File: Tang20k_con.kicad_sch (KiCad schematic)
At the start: 1 part

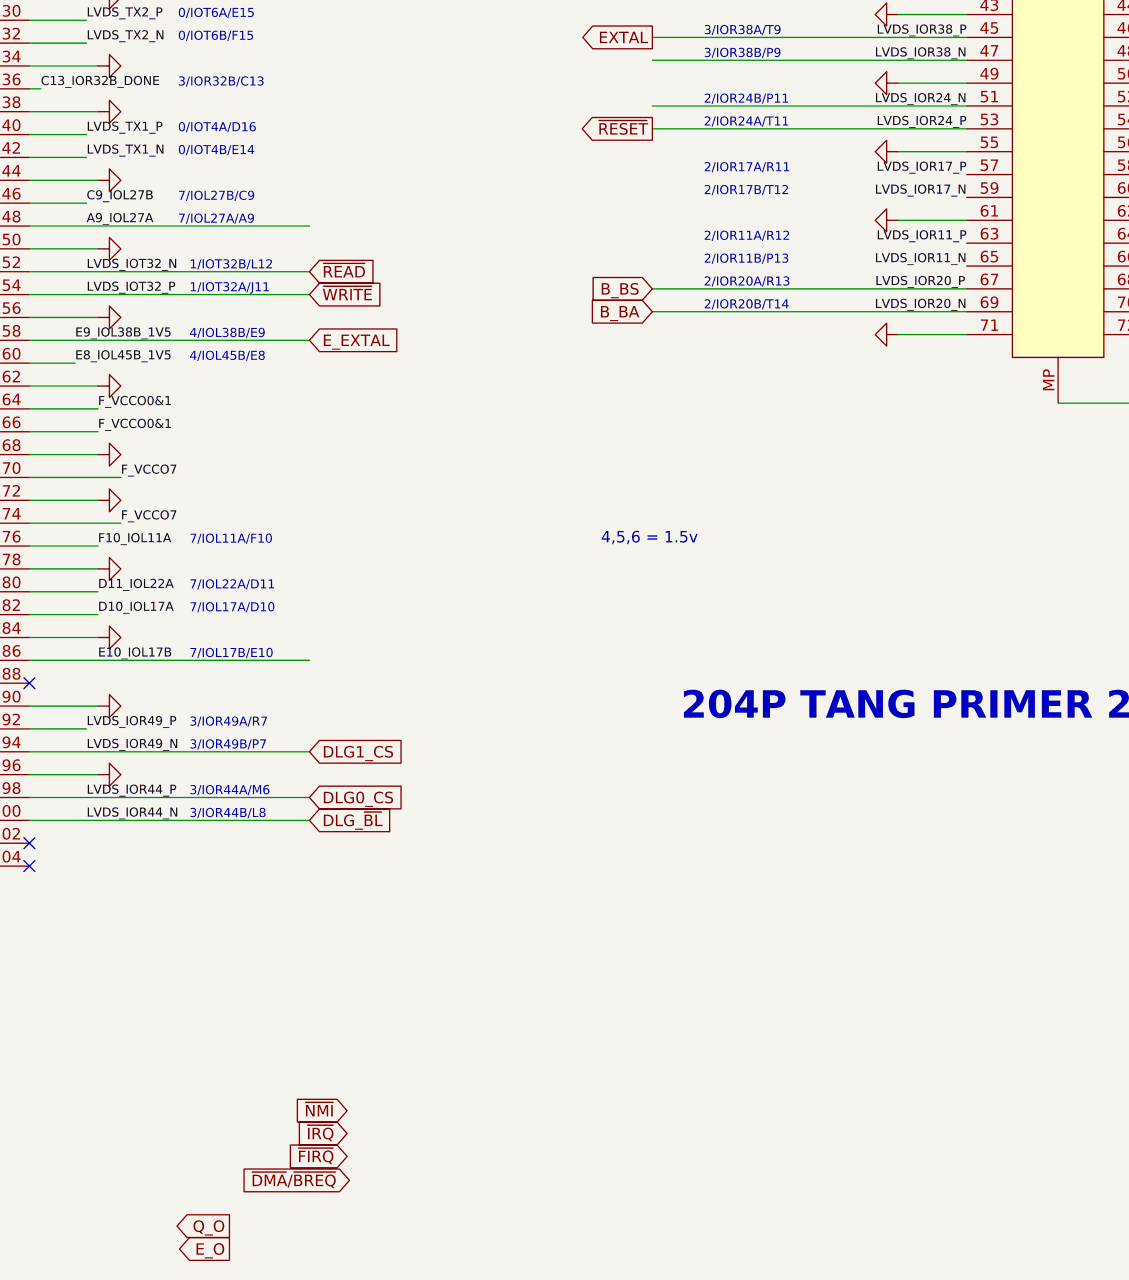
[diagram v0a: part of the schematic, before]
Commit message: WIP
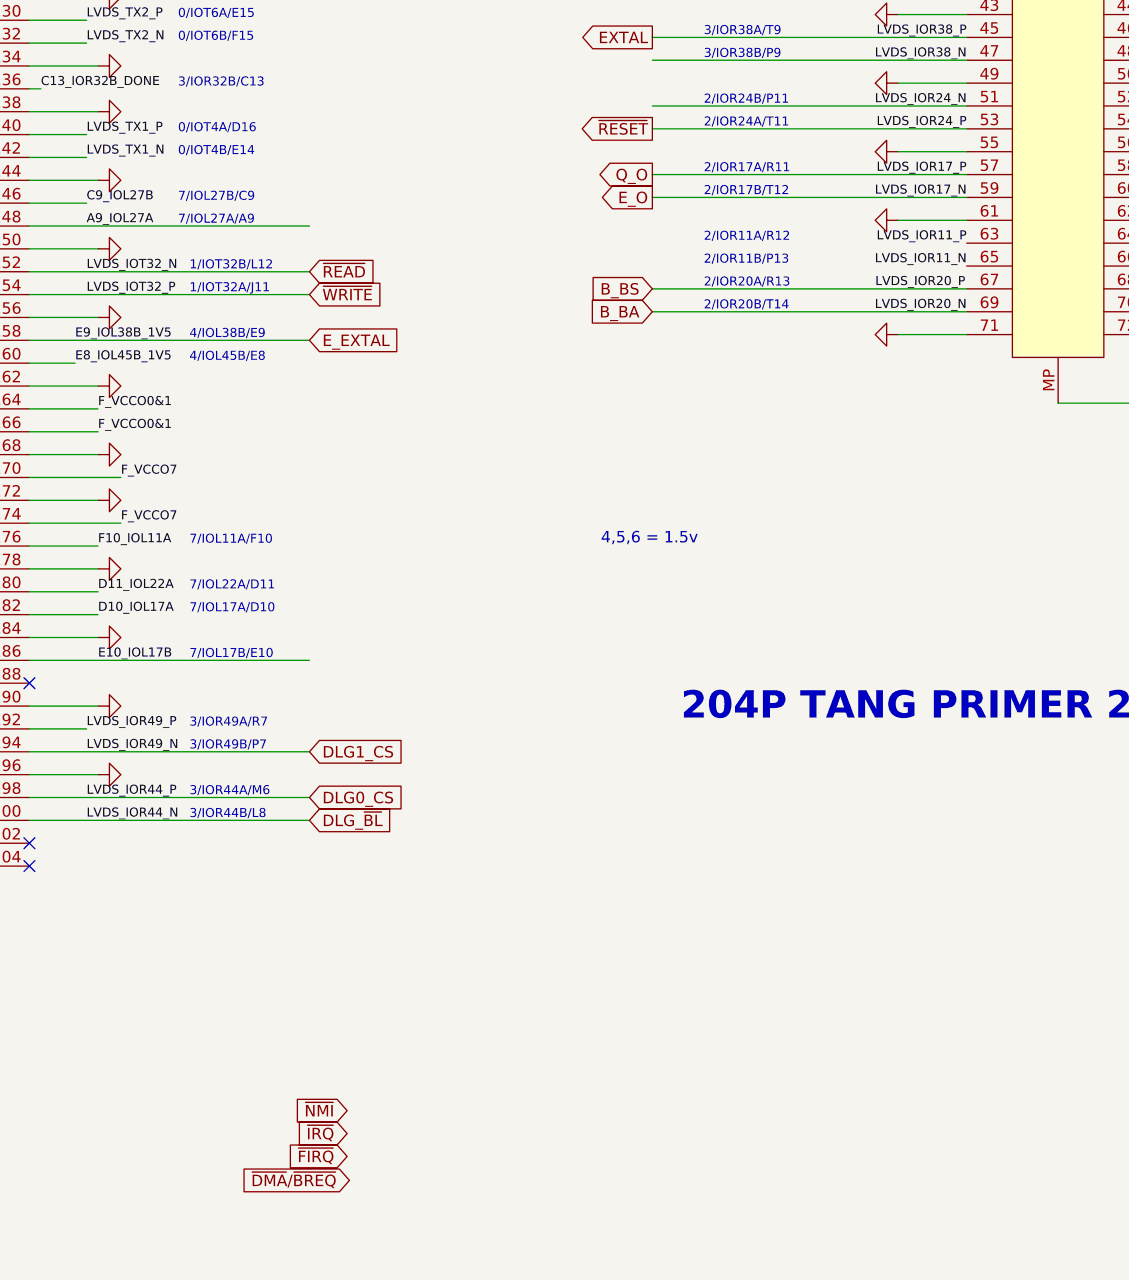
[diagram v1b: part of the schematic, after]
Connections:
- net LVDS_IOR17_N is gone; now on net E_O: TANG_PRIMER_20K_1.59
- net LVDS_IOR17_P is gone; now on net Q_O: TANG_PRIMER_20K_1.57
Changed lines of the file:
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@@
+    (stroke (width 0) (type default))
+  )
+  (wire (pts (xy 176.53 113.665) (xy 211.455 113.665))
     (stroke (width 0) (type default))
   )
@@
   )
   (wire (pts (xy 138.43 124.46) (xy 107.315 124.46))
+    (stroke (width 0) (type default))
+  )
+  (wire (pts (xy 176.53 116.205) (xy 211.455 116.205))
     (stroke (width 0) (type default))
   )
@@
     )
   )
-  (global_label "Q_O" (shape output) (at 129.54 230.505 180) (fields_autoplaced)
-    (effects (font (size 1.27 1.27)) (justify right))
-    (property "Intersheetrefs" "${INTERSHEET_REFS}" (at 123.0056 230.505 0)
+  (global_label "Q_O" (shape output) (at 176.53 113.665 180) (fields_autoplaced)
+    (effects (font (size 1.27 1.27)) (justify right))
+    (property "Intersheetrefs" "${INTERSHEET_REFS}" (at 169.9956 113.665 0)
       (effects (font (size 1.27 1.27)) (justify right) hide)
     )
@@
     )
   )
-  (global_label "E_O" (shape output) (at 129.54 233.045 180) (fields_autoplaced)
-    (effects (font (size 1.27 1.27)) (justify right))
-    (property "Intersheetrefs" "${INTERSHEET_REFS}" (at 123.1871 233.045 0)
-      (effects (font (size 1.27 1.27)) (justify right) hide)
-    )
+  (global_label "E_O" (shape output) (at 176.53 116.205 180) (fields_autoplaced)
+    (effects (font (size 1.27 1.27)) (justify right))
+    (property "Intersheetrefs" "${INTERSHEET_REFS}" (at 170.1771 116.205 0)
+      (effects (font (size 1.27 1.27)) (justify right) hide)
+    )

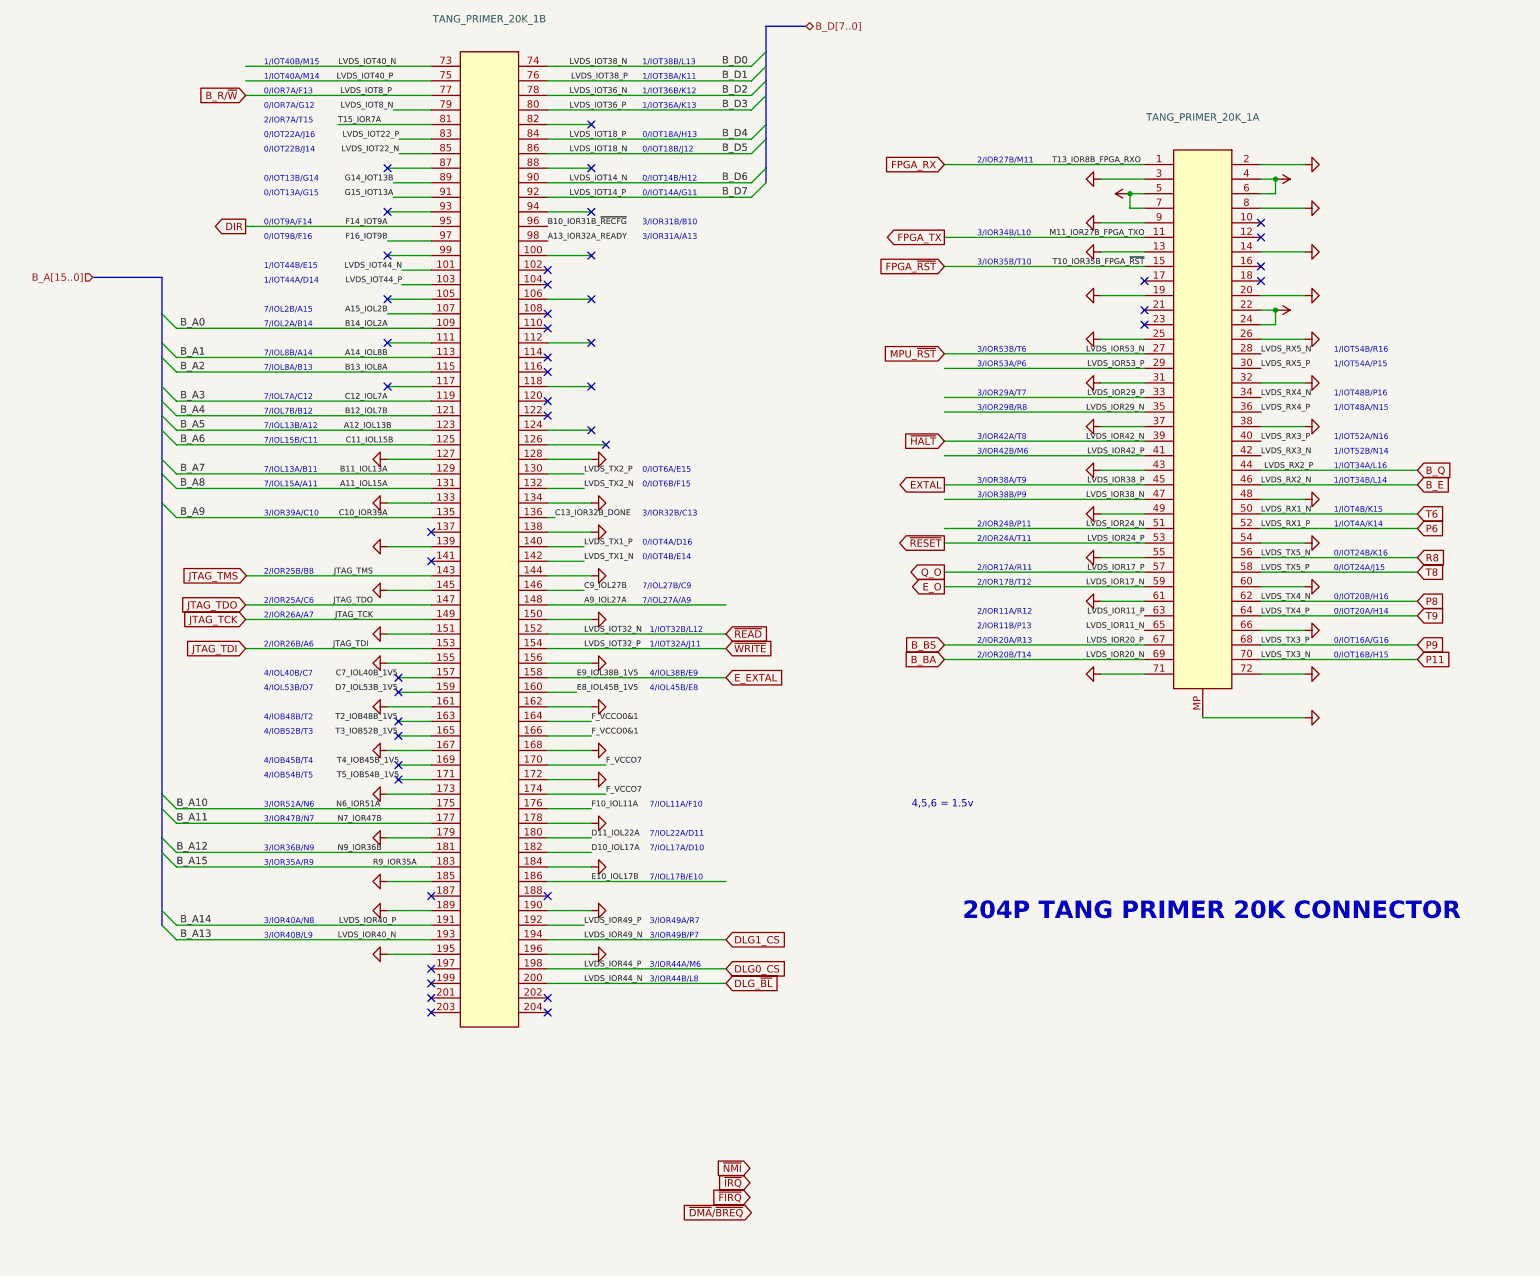
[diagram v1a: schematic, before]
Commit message: WIP
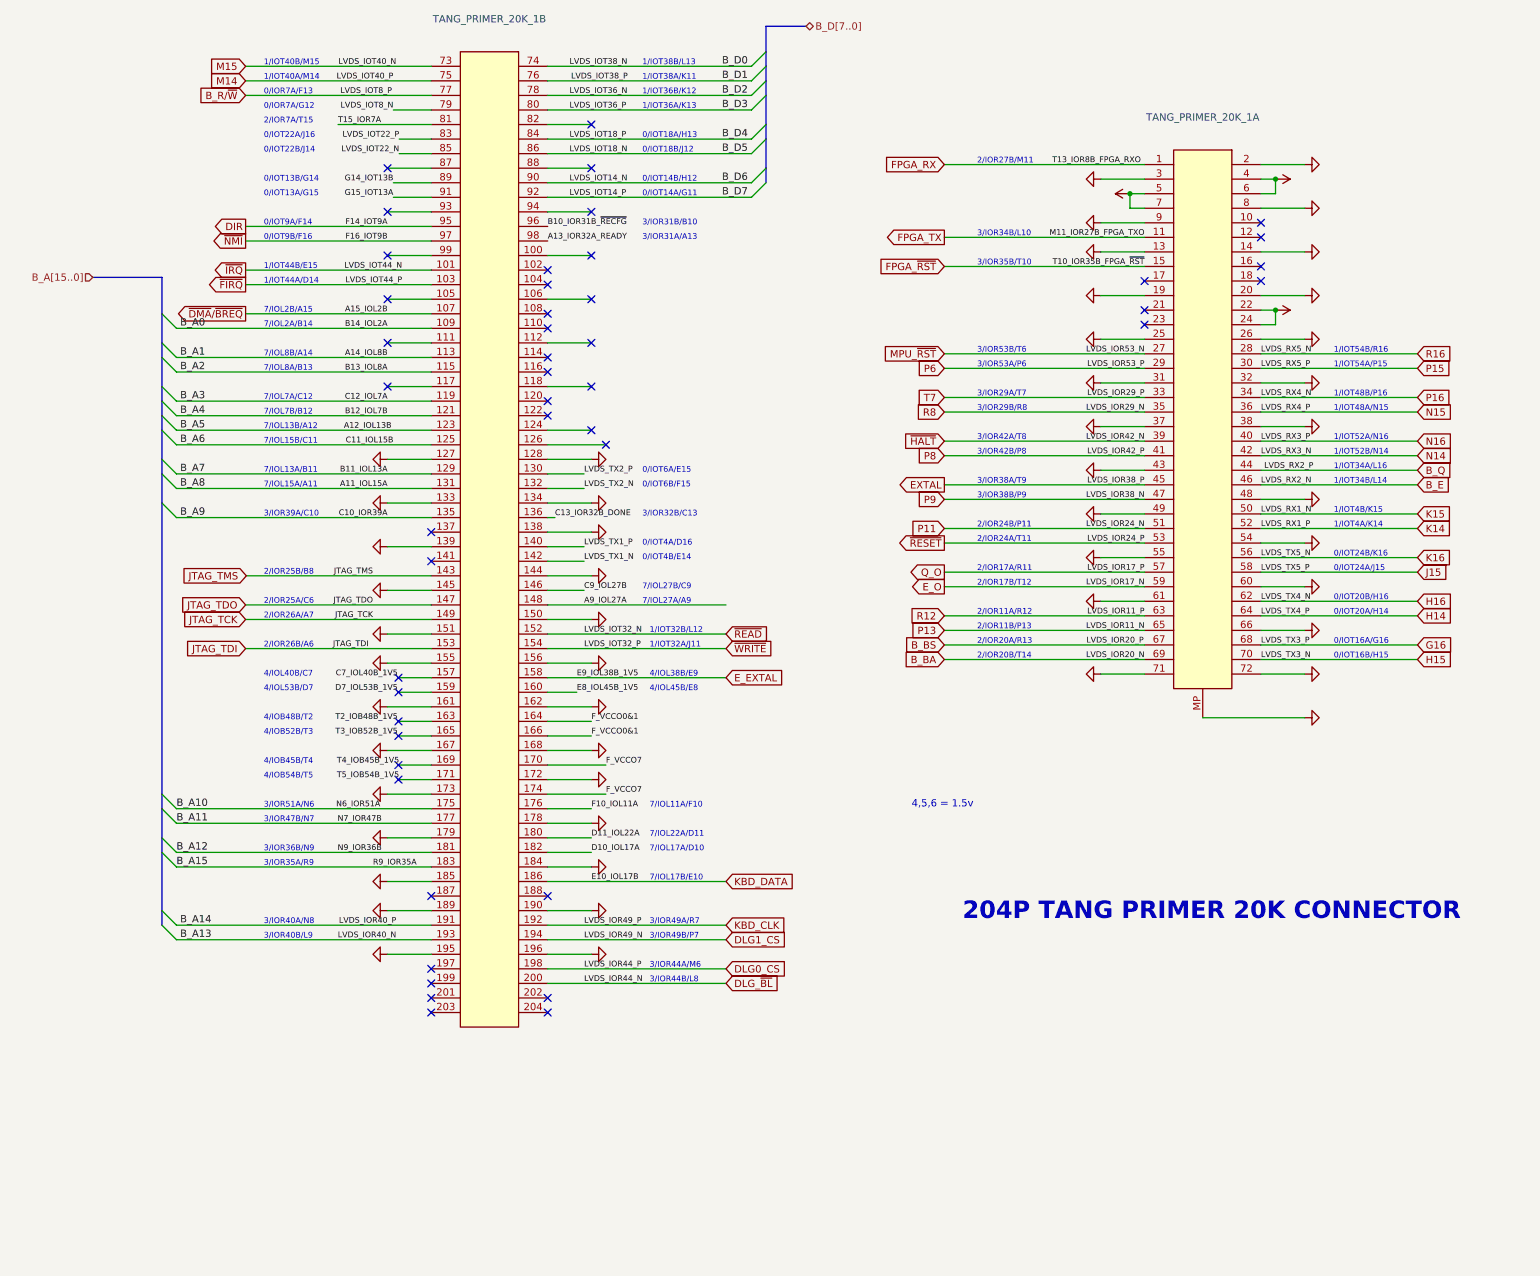
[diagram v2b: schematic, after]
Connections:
- net A15_IOL2B is gone; now on net ~{DMA}/~{BREQ}: TANG_PRIMER_20K_1.107
- net F16_IOT9B is gone; now on net ~{NMI}: TANG_PRIMER_20K_1.97
- net LVDS_IOR24_N is gone; now on net P11: TANG_PRIMER_20K_1.51
- net LVDS_IOR29_N is gone; now on net R8: TANG_PRIMER_20K_1.35
- net LVDS_IOR38_N is gone; now on net P9: TANG_PRIMER_20K_1.47
- net LVDS_IOR42_P is gone; now on net P8: TANG_PRIMER_20K_1.41
- net LVDS_IOR53_P is gone; now on net P6: TANG_PRIMER_20K_1.29
- net LVDS_IOT44_N is gone; now on net ~{IRQ}: TANG_PRIMER_20K_1.101
- net LVDS_IOT44_P is gone; now on net ~{FIRQ}: TANG_PRIMER_20K_1.103
- net P11: no longer TANG_PRIMER_20K_1.70
- net P6: no longer TANG_PRIMER_20K_1.52
- net P8: no longer TANG_PRIMER_20K_1.62
- net P9: no longer TANG_PRIMER_20K_1.68
- net R8: no longer TANG_PRIMER_20K_1.56
- net E10_IOL17B renamed KBD_DATA
- net LVDS_IOR11_N renamed P13
- net LVDS_IOR11_P renamed R12
- net LVDS_IOR29_P renamed T7
- net LVDS_IOR49_P renamed KBD_CLK
- net LVDS_IOT40_N renamed M15
- net LVDS_IOT40_P renamed M14
- net LVDS_RX3_N renamed N14
- net LVDS_RX3_P renamed N16
- net LVDS_RX4_N renamed P16
- net LVDS_RX4_P renamed N15
- net LVDS_RX5_N renamed R16
- net LVDS_RX5_P renamed P15
- net T6 renamed K15
- net T8 renamed J15
- net T9 renamed H14
- new net G16: TANG_PRIMER_20K_1.68
- new net H15: TANG_PRIMER_20K_1.70
- new net H16: TANG_PRIMER_20K_1.62
- new net K14: TANG_PRIMER_20K_1.52
- new net K16: TANG_PRIMER_20K_1.56
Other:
- note added: "3/IOR42B/P8"
- note removed: "3/IOR42B/M6"
